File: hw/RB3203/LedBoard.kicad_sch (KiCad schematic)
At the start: 22 parts

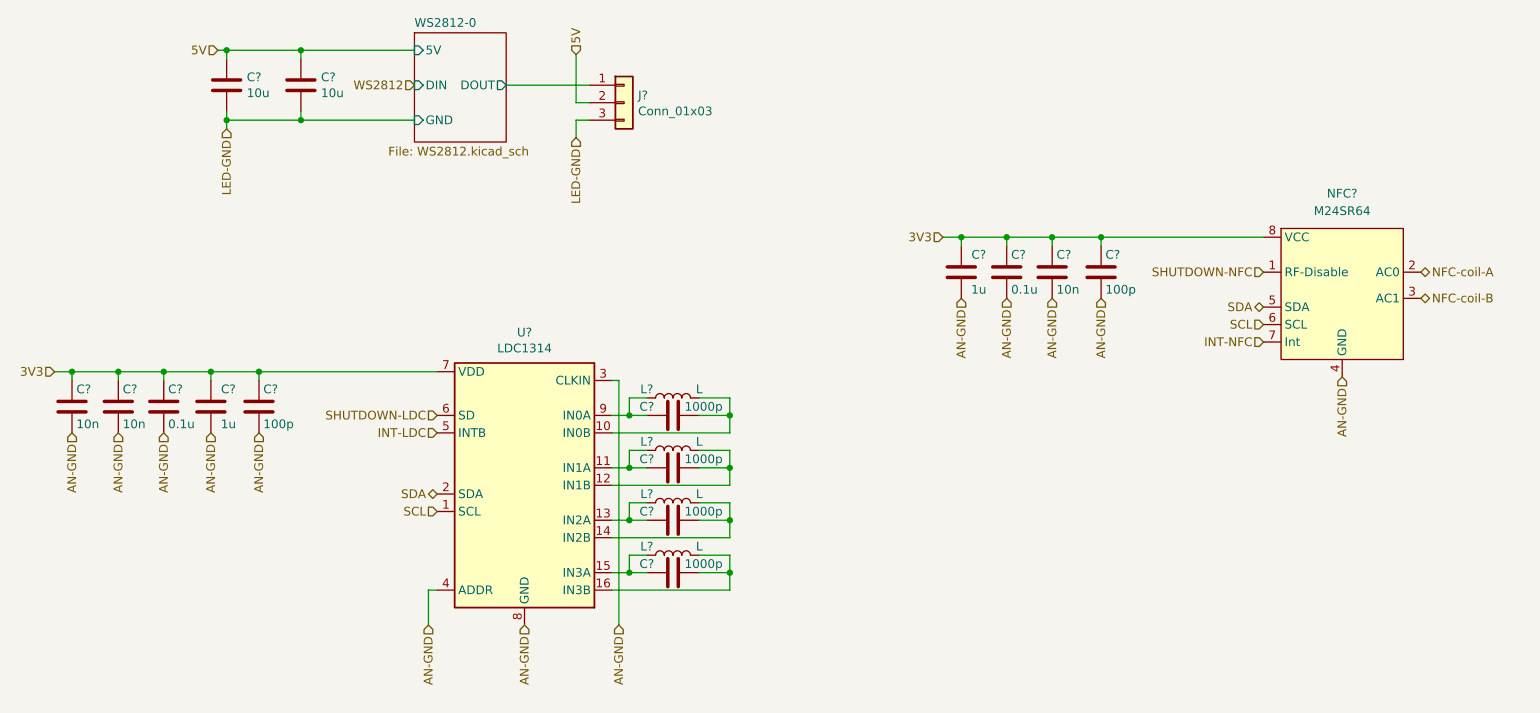
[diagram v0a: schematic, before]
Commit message: Wip
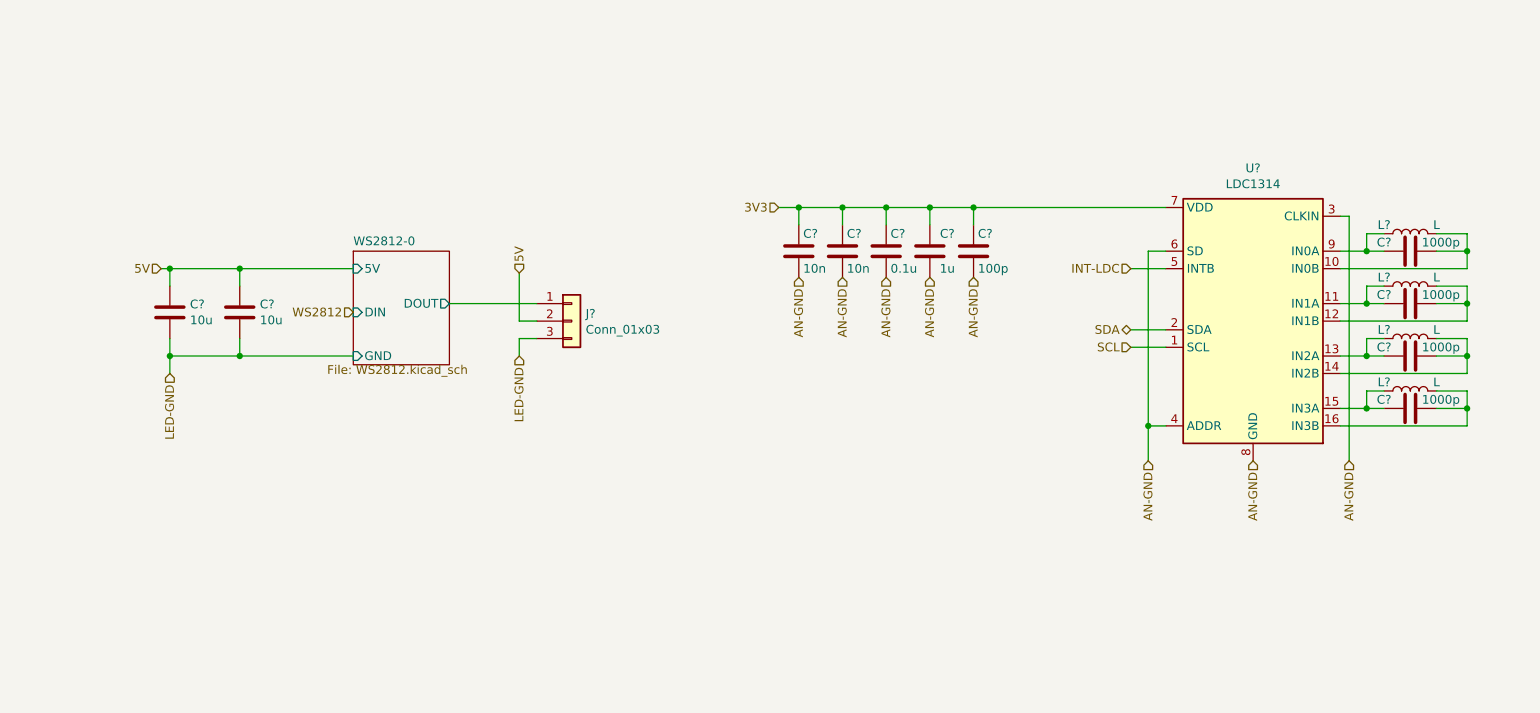
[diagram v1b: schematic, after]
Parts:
- removed C?: 1u, Capacitor_SMD:C_0402_1005Metric, symbol B.B-rescue:C-Device-B.B-rescue
- removed C?: 10n, Capacitor_SMD:C_0402_1005Metric, symbol B.B-rescue:C-Device-B.B-rescue
- removed C?: 0.1u, Resistor_SMD:R_0402_1005Metric, symbol B.B-rescue:C-Device-B.B-rescue
- removed C?: 100p, Capacitor_SMD:C_0402_1005Metric, symbol B.B-rescue:C-Device-B.B-rescue
- removed NFC?: M24SR64, symbol RB3203-Lib:M24SR64
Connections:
- net SHUTDOWN-LDC is gone; now on net AN-GND: U?.6 (SD)
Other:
- moved on the sheet: C?, J?, L?, U?
